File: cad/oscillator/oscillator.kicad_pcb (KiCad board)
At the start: 2 copper layers, 105.5 x 66.5 mm, 11 parts, among them U1 LM7805_TO220, U2 74LS00, Y1 DIL-14 VCXO 10Mhz

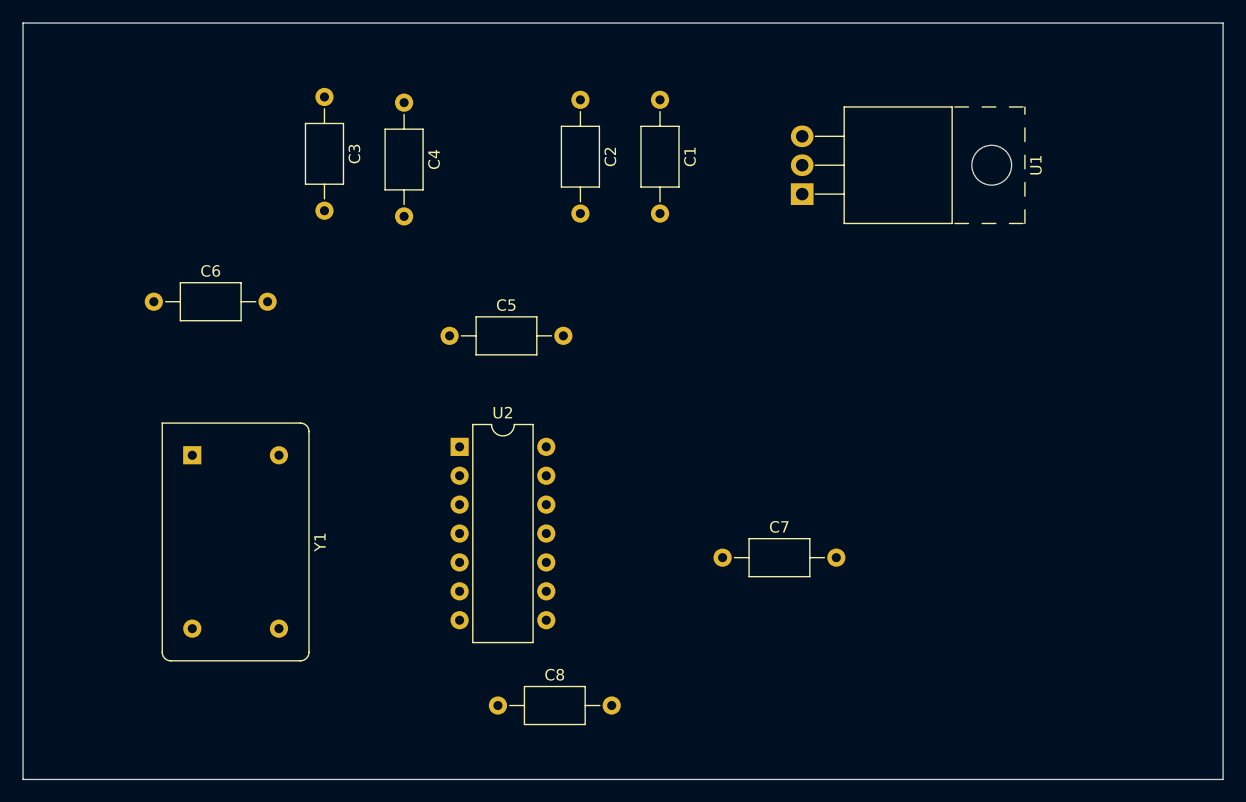
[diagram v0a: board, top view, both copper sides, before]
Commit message: Oscillator Updates
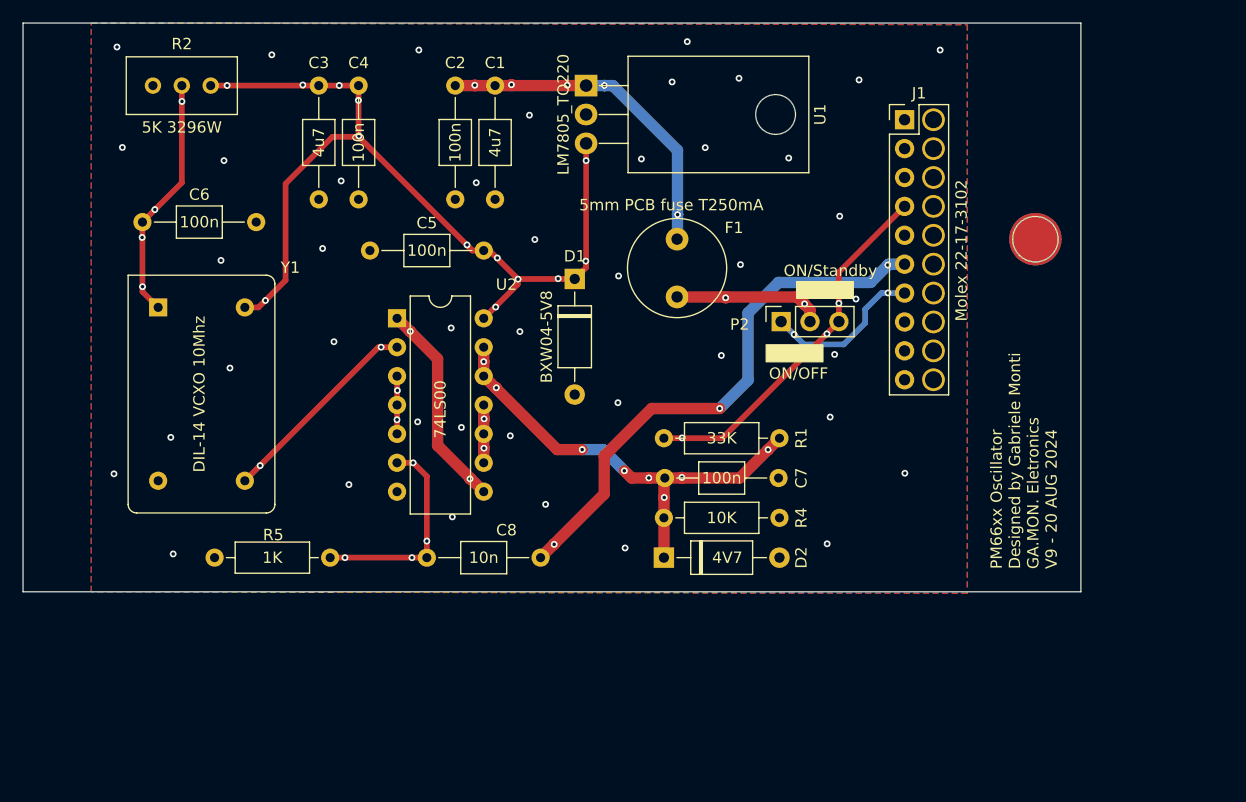
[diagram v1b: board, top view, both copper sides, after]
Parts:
- added D1: BXW04-5V8, Diode_THT:D_A-405_P10.16mm_Horizontal, F.Cu at (142.5, 87.5)
- added D2: 4V7, Diode_THT:D_A-405_P10.16mm_Horizontal, F.Cu at (150.3, 112.0)
- added F1: 5mm PCB fuse T250mA, Fuse:Fuse_Littelfuse_372_D8.50mm, F.Cu at (151.5, 84.0)
- added J1: Molex 22-17-3102, Connector_PinHeader_2.54mm:PinHeader_2x10_P2.54mm_Vertical, F.Cu at (171.5, 73.5)
- added P2: Supply-Mode Jumper, Connector_PinSocket_2.54mm:PinSocket_1x03_P2.54mm_Vertical, F.Cu at (160.6, 91.2)
- added R1: 33K, Resistor_THT:R_Axial_DIN0207_L6.3mm_D2.5mm_P10.16mm_Horizontal, F.Cu at (150.3, 101.5)
- added R2: 5K 3296W, Potentiometer_THT:Potentiometer_Bourns_3296W_Vertical, F.Cu at (110.5, 70.5)
- added R4: 10K, Resistor_THT:R_Axial_DIN0207_L6.3mm_D2.5mm_P10.16mm_Horizontal, F.Cu at (150.3, 108.5)
- added R5: 1K, Resistor_THT:R_Axial_DIN0207_L6.3mm_D2.5mm_P10.16mm_Horizontal, F.Cu at (121.0, 112.0)
- C1, C2, C3, C4, C5, C6, C7, C8: footprint Capacitor_THT:C_Axial_L5.1mm_D3.1mm_P10.00mm_Horizontal -> Capacitor_THT:C_Axial_L3.8mm_D2.6mm_P10.00mm_Horizontal
- U1: footprint Package_TO_SOT_THT:TO-220-3_Horizontal_TabUp -> Package_TO_SOT_THT:TO-220-3_Horizontal_TabDown
- moved U1 21.3 mm to (143.5, 70.5), turned to -90 degrees
- moved C1 14.6 mm to (135.5, 70.5)
- moved C8 14.4 mm to (129.5, 112.0)
- moved Y1 13.3 mm to (105.9, 90.0)
- moved U2 12.6 mm to (126.9, 91.0)
- moved C2 11.1 mm to (132.0, 70.5)
- moved C5 10.3 mm to (124.5, 85.0)
- moved C7 8.65 mm to (150.4, 105.0)
- moved C6 7.07 mm to (104.5, 82.5)
- moved C4 4.27 mm to (123.5, 70.5)
- moved C3 1.12 mm to (120.0, 70.5)
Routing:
- net Net-(D1-K): track 0.00 -> 80.2 mm, vias 0 -> 13
- net Net-(J1-Pin_6): track 0.00 -> 48.1 mm, vias 0 -> 3
- net Net-(D2-K): track 0.00 -> 40.9 mm, vias 0 -> 8
- net Net-(J1-Pin_4): track 0.00 -> 32.2 mm, vias 0 -> 3
- net Net-(U1-VI): track 0.00 -> 29.9 mm, vias 0 -> 5
- net Net-(Y1-Vcontrol): track 0.00 -> 21.6 mm, vias 0 -> 4
- net Net-(C8-Pad1): track 0.00 -> 18.8 mm, vias 0 -> 4
- net Net-(U2-Pad1): track 0.00 -> 18.5 mm, vias 0 -> 2
- net Net-(Y1-OUT): track 0.00 -> 18.3 mm, vias 0 -> 2
- net Net-(J1-Pin_7): track 0.00 -> 14.3 mm, vias 0 -> 2
- net Net-(P2-C): track 0.00 -> 13.3 mm, vias 0 -> 2
- net Net-(U2-Pad10): track 0.00 -> 5.13 mm, vias 0 -> 2
- net Net-(U2-Pad3): track 0.00 -> 5.11 mm, vias 0 -> 2
- net GND: vias 0 -> 43
- added copper zone on B.Cu, net GND
- added copper zone on F.Cu, net GND
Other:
- board size 105.5 x 66.5 mm -> 93 x 50 mm
- board text added: "ON/OFF"
- board text added: "ON/Standby"
- board text added: "PM66xx Oscillator Designed by Gabriele Monti GA.MON. Eletronics V9 - 20 AUG 2024"
